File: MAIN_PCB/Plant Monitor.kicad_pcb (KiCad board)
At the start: 4 copper layers, 42.8 x 66.3 mm, 58 parts, among them J1 TYPE-C-31-M-12, J10 BME280 Terminals, J2 Motor 1, J3 Motor 2, J4 Grove Connector for Soil Mois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, J5 JST PH-2Pin, J6 Grove Connector for OLED Disp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, J8 Conn_01x15, Q1 AO3401A, SW1 SW_Push, SW2 SW_Push, U1 RP2040, U2 AP2112K-3.3, U3 DRV8833PWP, U4 W25Q16JVSS, U6 MCP73831-2-OT, X1 ABM8-272-T3

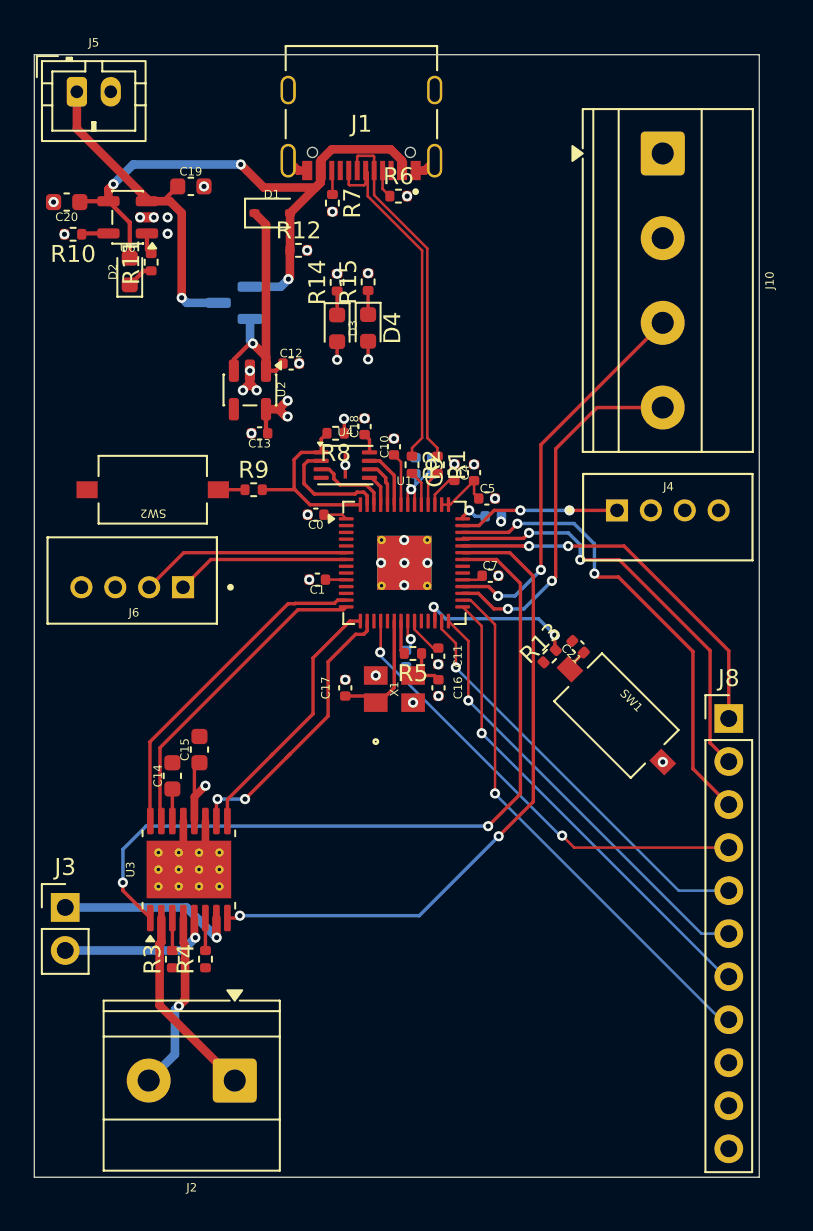
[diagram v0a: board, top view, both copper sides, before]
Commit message: Finished main PCB
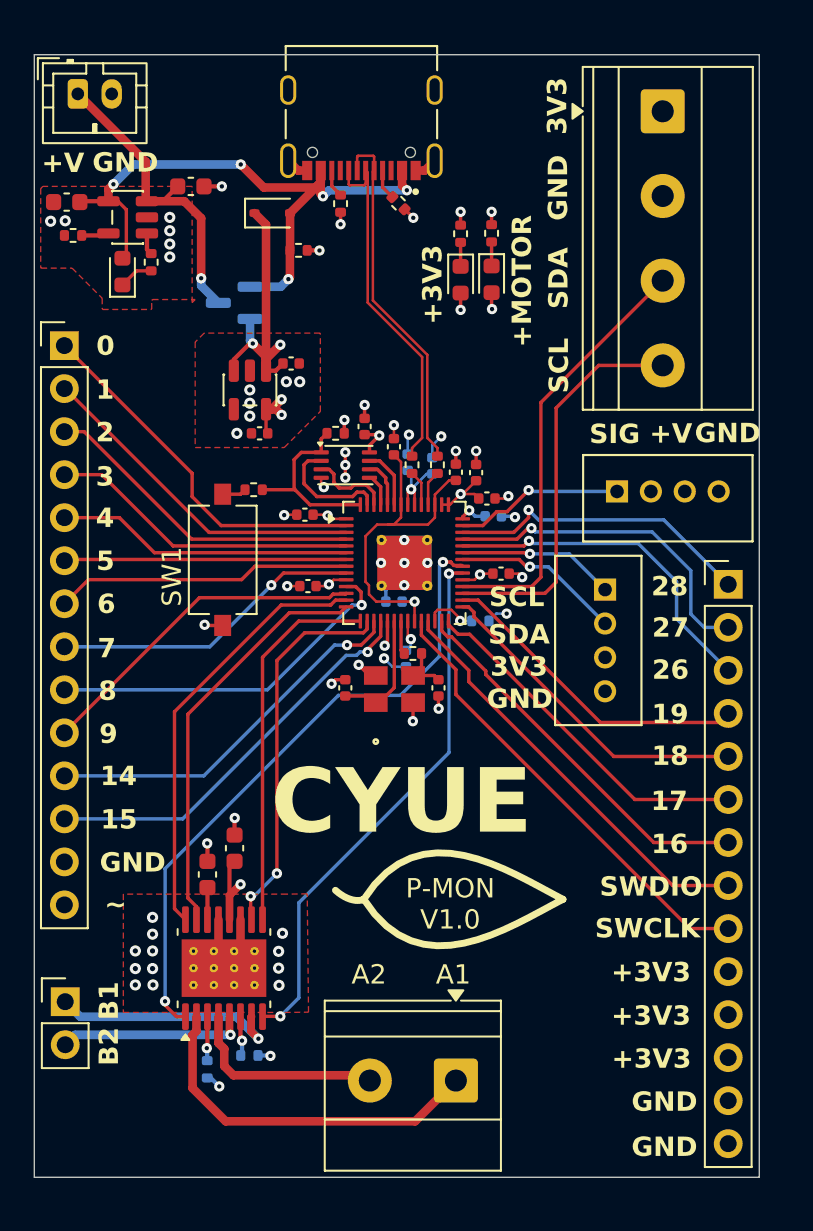
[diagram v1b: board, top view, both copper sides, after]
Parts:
- removed C21: 0.1uF, Capacitor_SMD:C_0402_1005Metric
- removed the J8 at (244.0, 99.6)
- removed the SW1 at (237.4, 99.5)
- added J6: Conn_01x14, Connector_PinHeader_2.54mm:PinHeader_1x14_P2.54mm_Vertical, F.Cu at (244.0, 91.7)
- added J7: Conn_01x14, Connector_PinHeader_2.54mm:PinHeader_1x14_P2.54mm_Vertical, F.Cu at (204.8, 77.6)
- C11, R13, R3, R4: moved to B.Cu
- moved J5 28.1 mm to (236.7, 95.0), turned to -90 degrees
- moved J2 13.1 mm to (227.9, 121.0)
- moved R15 7.83 mm to (230.0, 71.0)
- moved D3 7.83 mm to (228.2, 73.7)
- moved D4 7.83 mm to (230.0, 73.7)
- moved R14 7.83 mm to (228.2, 71.0)
- moved R3 6.82 mm to (213.2, 120.3)
- moved R4 6.25 mm to (215.7, 119.5), turned to 180 degrees
- moved U3 6.18 mm to (214.2, 114.4)
- moved C14 6.18 mm to (213.2, 108.8)
- moved C15 6.18 mm to (214.8, 107.3)
- moved SW1 5.85 mm to (214.1, 90.3), turned to -90 degrees
- moved J3 5.57 mm to (204.8, 116.4)
- moved R13 4.59 mm to (229.3, 93.9), turned to 180 degrees
- moved C11 4.15 mm to (224.2, 92.7), turned to 180 degrees
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- renumbered J6 to J5, J5 to J8, J10 to J9, SW2 to SW1, U6 to U5
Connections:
- net /RUN renamed Net-(U1-RUN)
- U1 pad 24: unconnected-(U1-SWCLK-Pad24) -> /SWCLK
- U1 pad 25: unconnected-(U1-SWDIO-Pad25) -> /SWDIO
- U1 pad 34: /GPIO22 -> /nFAULT
- U1 pad 35: /GPIO23 -> /nSLEEP
- U1 pad 36: /nSLEEP -> /OLED_SDA
- U1 pad 37: /nFAULT -> /OLED_SCL
- U1 pad 38: /GPIO28/ADC0 -> /GPIO26/ADC0
- U1 pad 40: /GPIO27/ADC2 -> /GPIO28/ADC2
- U1 pad 6: /OLED_SDA -> /GPIO4
- U1 pad 7: /OLED_SCL -> /GPIO5
- U4 pad 9: (no net) -> GND
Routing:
- net /GPIO27/ADC2: track 27.9 -> 0.00 mm, vias 2 -> 0
- net /SWCLK: track 0.00 -> 27.0 mm
- net /SWDIO: track 0.00 -> 24.9 mm
- net GND: track 11.2 -> 34.9 mm, vias 38 -> 61
- net /GPIO14: track 0.00 -> 22.4 mm, vias 0 -> 1
- net /GPIO28/ADC0: track 22.3 -> 0.00 mm, vias 2 -> 0
- net /GPIO0: track 0.00 -> 21.8 mm
- net /GPIO8: track 0.00 -> 21.4 mm, vias 0 -> 1
- net /GPIO26/ADC0: track 0.00 -> 20.3 mm, vias 0 -> 1
- net /GPIO1: track 0.00 -> 20.2 mm
- net /GPIO9: track 0.00 -> 20.0 mm
- net /GPIO2: track 0.00 -> 19.3 mm
- net /GPIO7: track 0.00 -> 18.4 mm, vias 0 -> 1
- net /GPIO3: track 0.00 -> 18.4 mm
- net /GPIO28/ADC2: track 0.00 -> 18.3 mm, vias 0 -> 1
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- added copper zone on In2.Cu, net +3V3
- added copper zone on In3.Cu, net /+MOTORVOLTAGE
- added copper zone on F.Cu, net GND
- added copper zone on In4.Cu, net GND
- removed copper zone on In2.Cu, net /+MOTORVOLTAGE
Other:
- copper layers 4 -> 6
- board text added: "+3V3"
- board text added: "+MOTOR"
- board text added: "+V"
- board text added: "0"
- board text added: "1"
- board text added: "14"
- board text added: "15"
- board text added: "16"
- board text added: "17"
- board text added: "18"
- board text added: "19"
- board text added: "2"
- board text added: "26"
- board text added: "27"
- board text added: "28"
- board text added: "3"
- board text added: "3V3"
- board text added: "4"
- board text added: "5"
- board text added: "6"
- board text added: "7"
- board text added: "8"
- board text added: "9"
- board text added: "A1"
- board text added: "A2"
- board text added: "All vias that are in pads and have a total diameter of 24 mils and hole diameter 10 mils should be filled with epoxy and capped over (IPC-4761 Type VII via) All vias within copper pours should also be filled with epoxy for thermal conductivity"
- board text added: "B1"
- board text added: "B2"
- board text added: "CYUE"
- board text added: "GND"
- board text added: "P-MON V1.0"
- board text added: "SCL"
- board text added: "SDA"
- board text added: "SIG"
- board text added: "SWCLK"
- board text added: "SWDIO"
- board text added: "~"
